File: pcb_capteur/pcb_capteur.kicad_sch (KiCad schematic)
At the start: 22 parts, among them P1 Power, P2 Analog, P3 Digital, P4 Digital, P5 CONN_01X01, P6 CONN_01X01, P7 CONN_01X01, P8 CONN_01X01, U1 OLED-I2C, U2 LTC1050, U3 HC-05, U4 KY-040

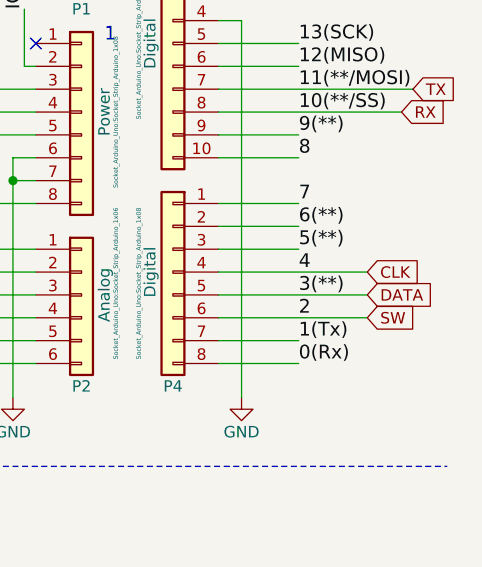
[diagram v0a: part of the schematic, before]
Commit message: Fourth commit
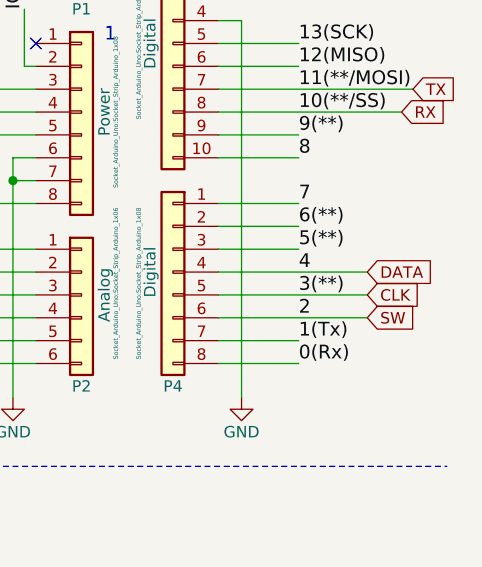
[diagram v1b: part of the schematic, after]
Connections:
- net CLK: now also P4.5 (Pin_5); no longer P4.4 (Pin_4)
- net DATA: now also P4.4 (Pin_4); no longer P4.5 (Pin_5)
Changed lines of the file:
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@@
-    )
-  )
-  (global_label "DATA" (shape input) (at 275.59 68.58 0) (fields_autoplaced)
-    (effects (font (size 1.27 1.27)) (justify left))
-    (property "Intersheet References" "${INTERSHEET_REFS}" (id 0) (at 282.6084 68.5006 0)
-      (effects (font (size 1.27 1.27)) (justify left) hide)
     )
   )
@@
     )
   )
-  (global_label "CLK" (shape input) (at 275.59 66.04 0) (fields_autoplaced)
-    (effects (font (size 1.27 1.27)) (justify left))
-    (property "Intersheet References" "${INTERSHEET_REFS}" (id 0) (at 281.7617 65.9606 0)
-      (effects (font (size 1.27 1.27)) (justify left) hide)
-    )
-  )
   (global_label "IN+" (shape input) (at 110.49 54.61 180) (fields_autoplaced)
     (effects (font (size 1.27 1.27)) (justify right))
     (property "Intersheet References" "${INTERSHEET_REFS}" (id 0) (at 104.3788 54.5306 0)
       (effects (font (size 1.27 1.27)) (justify right) hide)
+    )
+  )
+  (global_label "CLK" (shape input) (at 275.59 68.58 0) (fields_autoplaced)
+    (effects (font (size 1.27 1.27)) (justify left))
+    (property "Intersheet References" "${INTERSHEET_REFS}" (id 0) (at 281.7617 68.5006 0)
+      (effects (font (size 1.27 1.27)) (justify left) hide)
     )
   )
@@
     )
   )
+  (global_label "DATA" (shape input) (at 275.59 66.04 0) (fields_autoplaced)
+    (effects (font (size 1.27 1.27)) (justify left))
+    (property "Intersheet References" "${INTERSHEET_REFS}" (id 0) (at 282.6084 65.9606 0)
+      (effects (font (size 1.27 1.27)) (justify left) hide)
+    )
+  )
